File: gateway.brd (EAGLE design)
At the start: 48 x 42 mm, 72 parts, among them IC2 24AA00OT, J1 MAGJACK, Q3 BC817, U3 TPD4E002DRLR, U5 TPD4E002DRLR, U6 TPD4E002DRLR, U7 TPD4E002DRLR, U8 74LVC1G04GW, Y2 16MHz

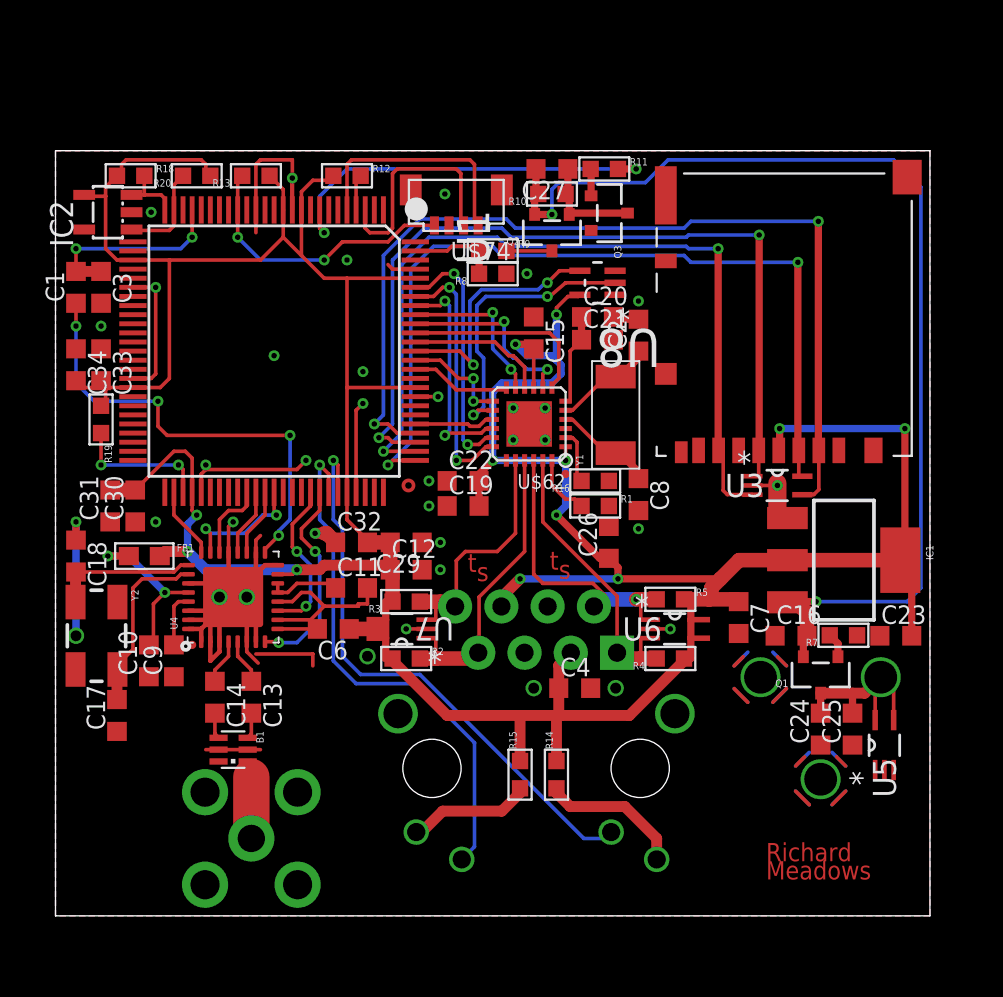
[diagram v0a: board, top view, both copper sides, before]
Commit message: Version 6
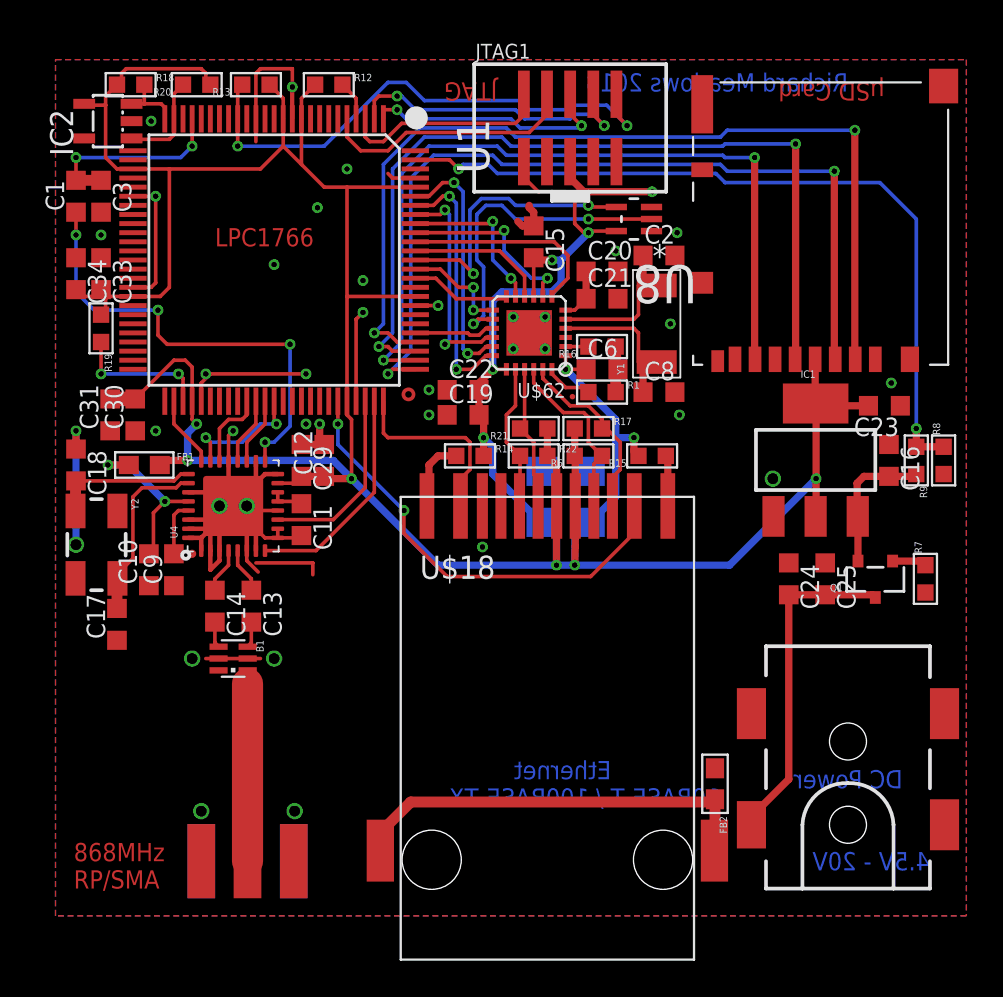
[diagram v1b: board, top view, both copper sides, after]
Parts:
- removed C26: 470pF, resistor:C0603K
- removed C27: 100pF, resistor:C0603K
- removed C32: 10nF, resistor:C0603K
- removed C7: 100nF, resistor:C0603K
- removed CN1: (no value), microbuilder:DCJACK_2MM_PTH2
- removed Q2: (no value), microbuilder:SOT23-R
- removed Q3: BC817, microbuilder:SOT23-R
- removed R10: 100K, microbuilder:0603-MINI
- removed R11: 2.2K, microbuilder:0603-MINI
- removed R2, R3, R4, R5: 49.9R, microbuilder:0603-MINI
- removed U$74: SM04B-SURS-TF, con-jst:SM04B-SURS-TF
- removed U3, U5, U6, U7: TPD4E002DRLR, TPD4E002:SOT50P280X60-5N
- removed X1: (no value), microbuilder:SMA90_DIP
- added C5: 100nF, resistor:C1206
- added FB2: (no value), microbuilder:0603
- added J$1: SMA_EDGE, SparkFun-Connectors:SMA-EDGE
- added JTAG1: (no value), microbuilder_v3:2X05_1.27MM_SMT
- added R17, R21, R22, R6: 49.9R, microbuilder:0603-MINI
- added U$18: J3011TIGHT, J3011:J3011_TIGHT
- C4: device resistor:C0603K -> resistor:C1206
- C6: value 100nF -> 470pF
- J1: value MAGJACK -> POWER_JACKSMD_2; device SparkFun:MAGJACK -> SparkFun:POWER_JACK_SMD_2
- moved R8 26.8 mm to (48.8, 25.0), turned to 90 degrees
- moved R9 25.9 mm to (47.2, 25.0), turned to 270 degrees
- moved C6 20.5 mm to (30.0, 30.0), turned to 0 degrees
- moved R15 18.9 mm to (32.8, 25.2), turned to 180 degrees
- moved R14 18.1 mm to (22.8, 25.2), turned to 0 degrees
- moved C23 12.6 mm to (45.5, 28.0), turned to 180 degrees
- moved J1 12.1 mm to (43.5, 5.00), flipped to the top, turned to 90 degrees
- moved C16 11.0 mm to (45.8, 25.0), turned to 270 degrees
- moved C4 10.6 mm to (26.8, 23.0), flipped to the bottom, turned to 90 degrees
- moved C24 8.43 mm to (40.2, 18.5), turned to 270 degrees
- moved C25 8.39 mm to (42.2, 18.5), turned to 270 degrees
- moved C12 7.50 mm to (14.8, 25.0), turned to 90 degrees
- moved R16 7.38 mm to (30.0, 31.2)
- moved C29 7.30 mm to (13.5, 25.0), turned to 270 degrees
- moved R1 6.26 mm to (30.0, 28.8)
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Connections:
- removed net N$6: U1.48
- removed net N$7: U1.49
- removed net PWR_MON_EN: R11.2, U1.8
- removed net PWR_MON_EN_SW: C27.1, Q2.1, Q3.3, R10.1
- removed net PWR_MON_SW: Q2.3, R9.2
- removed net Q3RES: Q3.1, R11.1
- removed net SD_EN: U1.9
- new net CGND: FB2.2, U$18.PAD1, U$18.PAD2
- new net TDI: JTAG1.8, U1.2
- new net TDO_SWO: JTAG1.6, U1.1
- net !RESET!: now also JTAG1.10; no longer U$74.4
- net 3.3V: now also C5.1, JTAG1.1, R17.1, R21.1, R22.2, R6.2, U$18.5, U$18.6; no longer C26.1, C32.2, C7.1, J1.3, J1.6, R2.1, R3.2, R4.1, R5.2, U6.4, U6.5, U7.4, U7.5
- net GLED: now also U$18.11, U1.75; no longer J1.10, U1.70
- net GLED+: now also U$18.12; no longer J1.9
- net GND: now also C5.2, FB2.1, J$1.GND@0, J$1.GND@1, J$1.GND@2, J$1.GND@3, J1.GND, J1.P$4, JTAG1.3, JTAG1.5, JTAG1.9, U$18.10; no longer C26.2, C32.1, C7.2, CN1.GND, CN1.GNDBREAK, Q3.2, U$74.3, U$74.GND1, U$74.GND2, U3.2, U5.1, U5.2, U5.3, U6.2, U7.2, X1.GND1, X1.GND2, X1.GND3, X1.GND4
- net PWR: now also J1.VIN0; no longer CN1.PWR, U5.4, U5.5
- net RADIORST: now also U1.74; no longer U1.68
- net RD+: now also R21.2, U$18.7, U$62.21; no longer J1.1, R4.2, U$62.23, U6.3
- net RD-: now also R22.1, U$18.8, U$62.20; no longer J1.2, R5.1, U$62.22, U6.1
- net RPWR: now also R9.2; no longer C27.2, Q2.2, R10.2
- net SD_CLK: no longer U3.1
- net SD_CS: no longer U3.4
- net SD_MISO: no longer U3.3
- net SD_MOSI: no longer U3.5
- net SLP_TR: now also U1.73; no longer U1.67
- net TCK_SWDCLK: now also JTAG1.4; no longer U$74.1
- net TD+: now also R17.2, U$18.3, U$62.23; no longer J1.7, R2.2, U$62.21, U7.1
- net TD-: now also R6.1, U$18.4, U$62.22; no longer J1.8, R3.1, U$62.20, U7.3
- net TMS_SWDIO: now also JTAG1.2; no longer U$74.2
- net UNBAL: now also J$1.SIG; no longer X1.ANTENNA
- net YLED: now also U$18.2, U1.70; no longer J1.11, U1.69
- net YLED+: now also U$18.1; no longer J1.12
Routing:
- net RPWR: track 60.0 -> 7.75 mm, vias 2 -> 0
- net PWR_MON: track 4.96 -> 43.1 mm, vias 0 -> 2
- net CGND: track 0.00 -> 23.0 mm
- net PWR_MON_EN: track 22.5 -> 0.00 mm, vias 2 -> 0
- net GLED: track 31.9 -> 10.4 mm, vias 1 -> 0
- net TDI: track 0.00 -> 16.6 mm, vias 0 -> 2
- net 3.3V: track 226.9 -> 210.6 mm
- net !RESET!: track 15.6 -> 29.5 mm
- net TDO_SWO: track 0.00 -> 13.8 mm, vias 0 -> 2
- net RD-: track 16.9 -> 8.03 mm, vias 1 -> 0
- net PWR: track 11.0 -> 19.5 mm
- net RD+: track 16.1 -> 8.01 mm
- net TD+: track 17.0 -> 10.2 mm
- net UNBAL: track 4.28 -> 10.5 mm
- net PWR_MON_EN_SW: track 6.02 -> 0.00 mm
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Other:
- board outline removed
- board text added: "10BASE-T / 100BASE-TX"
- board text added: "4.5V - 20V"
- board text added: "868MHz"
- board text added: "DC Power"
- board text added: "Ethernet"
- board text added: "JTAG"
- board text added: "LPC1766"
- board text added: "RP/SMA"
- board text added: "Richard Meadows 2013"
- board text added: "µSD Card"
- board text removed: "Meadows"
- board text removed: "Richard"
- board text removed: "s"
- board text removed: "t"
